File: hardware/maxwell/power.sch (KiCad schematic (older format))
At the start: 30 parts, among them J7 Dynamo Input, J9 Battery, Q2 PSMN5R4-25YLD, Q3 NTR1P02T1, Q4 NTR1P02T1, Q5 NTR1P02T1, U10 MIC39102, U8 TLP188, U9 Buck Regulator

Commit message: Updating for manufacture.
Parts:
- removed C15: 100u, coddingtonbear:CP_Tantalum_Case-D_EIA-7343-31_Milling, symbol maxwell-rescue:CP-RESCUE-maxwell
- removed D2, D3: 18, adamgreig/agg-kicad/agg.pretty:DO-214AA-SMB, symbol maxwell-rescue:D_Zener-RESCUE-maxwell
- removed R34: 110k, coddingtonbear/coddingtonbear.pretty:0805_Milling, symbol maxwell-rescue:R-RESCUE-maxwell
- removed R35: 10k, coddingtonbear/coddingtonbear.pretty:0805_Milling, symbol maxwell-rescue:R-RESCUE-maxwell
- added D2: GS1M-LTP, mcous/kicad-lib/footprints/diode.pretty:DO-214AC, symbol pspice:DIODE
- added J18: Supercap, coddingtonbear/coddingtonbear.pretty:JST_XH_B02B-XH-A_02x2.50mm_Straight_LargePads, symbol maxwell-rescue:Conn_01x02-RESCUE-maxwell
- added Q6: NTR1P02T1, coddingtonbear/coddingtonbear.pretty:SOT-23_LargePads, symbol device:Q_PMOS_GSD
- added R15: 10k, coddingtonbear/coddingtonbear.pretty:0805_Milling, symbol maxwell-rescue:R-RESCUE-maxwell
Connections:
- net labels added: BATT_SOURCE_DISABLE, VCC
- net labels removed: DYNAMO_VOLTAGE
- wire segments 85 -> 87
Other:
- note added: "Tune to 5V"
- note removed: "Tune to 4V"
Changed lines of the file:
@@
-$EndComp
-$Comp
-L maxwell-rescue:D_Zener-RESCUE-maxwell D2
-U 1 1 5A1FF2A4
-P 2400 1050
-F 0 "D2" V 2354 1129 50  0000 L CNN
-F 1 "18" V 2445 1129 50  0000 L CNN
-F 2 "adamgreig/agg-kicad/agg.pretty:DO-214AA-SMB" H 2400 1050 50  0001 C CNN
-F 3 "" H 2400 1050 50  0001 C CNN
-	1    2400 1050
-	0    1    1    0
-$EndComp
-$Comp
-L maxwell-rescue:D_Zener-RESCUE-maxwell D3
-U 1 1 5A1FF2AB
-P 2400 1400
-F 0 "D3" V 2446 1321 50  0000 R CNN
-F 1 "18" V 2355 1321 50  0000 R CNN
-F 2 "adamgreig/agg-kicad/agg.pretty:DO-214AA-SMB" H 2400 1400 50  0001 C CNN
-F 3 "" H 2400 1400 50  0001 C CNN
-	1    2400 1400
-	0    -1   -1   0
 $EndComp
 $Comp
@@
 F 3 "" H 5150 1350 50  0001 C CNN
 	1    5150 1350
-	1    0    0    -1
-$EndComp
-$Comp
-L maxwell-rescue:CP-RESCUE-maxwell C15
-U 1 1 5A20260D
-P 3650 1600
-F 0 "C15" H 3768 1646 50  0000 L CNN
-F 1 "100u" H 3768 1555 50  0000 L CNN
-F 2 "coddingtonbear:CP_Tantalum_Case-D_EIA-7343-31_Milling" H 3688 1450 50  0001 C CNN
-F 3 "" H 3650 1600 50  0001 C CNN
-	1    3650 1600
-	1    0    0    -1
-$EndComp
-$Comp
-L maxwell-rescue:GND-RESCUE-maxwell #PWR040
-U 1 1 5A202661
-P 3650 1750
-F 0 "#PWR040" H 3650 1500 50  0001 C CNN
-F 1 "GND" H 3655 1577 50  0000 C CNN
-F 2 "" H 3650 1750 50  0001 C CNN
-F 3 "" H 3650 1750 50  0001 C CNN
-	1    3650 1750
 	1    0    0    -1
 $EndComp
@@
 ~BATT_CHARGING
 Text Notes 4400 1550 0    60   ~ 0
-Tune to 4V
+Tune to 5V
 $Comp
 L maxwell-rescue:C-RESCUE-maxwell C18
@@
 ~BATT_CHARGE_ENABLE
 $Comp
-L maxwell-rescue:R-RESCUE-maxwell R34
-U 1 1 5A27817C
-P 4150 850
-F 0 "R34" H 4220 896 50  0000 L CNN
-F 1 "110k" H 4220 805 50  0000 L CNN
-F 2 "coddingtonbear/coddingtonbear.pretty:0805_Milling" V 4080 850 50  0001 C CNN
-F 3 "" H 4150 850 50  0001 C CNN
-	1    4150 850
-	0    -1   -1   0
-$EndComp
-$Comp
-L maxwell-rescue:R-RESCUE-maxwell R35
-U 1 1 5A2781E1
-P 4500 850
-F 0 "R35" H 4570 896 50  0000 L CNN
-F 1 "10k" H 4570 805 50  0000 L CNN
-F 2 "coddingtonbear/coddingtonbear.pretty:0805_Milling" V 4430 850 50  0001 C CNN
-F 3 "" H 4500 850 50  0001 C CNN
-	1    4500 850
-	0    -1   -1   0
-$EndComp
-$Comp
-L maxwell-rescue:GND-RESCUE-maxwell #PWR046
-U 1 1 5A278243
-P 4650 850
-F 0 "#PWR046" H 4650 600 50  0001 C CNN
-F 1 "GND" H 4655 677 50  0000 C CNN
-F 2 "" H 4650 850 50  0001 C CNN
-F 3 "" H 4650 850 50  0001 C CNN
-	1    4650 850
-	0    -1   -1   0
-$EndComp
-Text GLabel 4400 650  2    60   Output ~ 0
-DYNAMO_VOLTAGE
-$Comp
 L maxwell-rescue:+BATT-RESCUE-maxwell #PWR043
 U 1 1 5A210C7A
@@
 $EndComp
 Wire Wire Line
-	2400 1250 2400 1200
-Wire Wire Line
-	1300 900  2400 900
-Wire Wire Line
-	1300 1550 2400 1550
-Wire Wire Line
 	3350 900  3350 950
-Connection ~ 2400 900
-Connection ~ 2400 1550
-Wire Wire Line
-	3650 1250 3650 1450
-Wire Wire Line
-	3650 1250 3800 1250
 Wire Wire Line
 	5600 1250 5650 1250
@@
 Connection ~ 10100 2150
 Wire Wire Line
-	5650 1600 5650 2000
+	5650 1600 5650 1900
 Wire Wire Line
 	5650 2000 5900 2000
@@
 Wire Wire Line
 	1500 3500 1350 3500
-Wire Wire Line
-	4000 850  3800 850
-Wire Wire Line
-	3800 850  3800 1250
-Connection ~ 3800 1250
-Wire Wire Line
-	4300 850  4350 850
-Wire Wire Line
-	4300 850  4300 650
-Wire Wire Line
-	4300 650  4400 650
 Wire Wire Line
 	5200 1250 5150 1250
@@
 DYNAMO_AC
 Wire Wire Line
-	2400 900  3350 900
-Wire Wire Line
-	2400 1550 3350 1550
-Wire Wire Line
 	5900 1250 6400 1250
 Wire Wire Line
@@
 Wire Wire Line
 	5900 2000 5900 2050
-Wire Wire Line
-	3800 1250 4200 1250
 Wire Wire Line
 	7350 1800 7450 1800
@@
 L maxwell-rescue:+BATT-RESCUE-maxwell #PWR037
 U 1 1 5A884C49
-P 4950 2850
-F 0 "#PWR037" H 4950 2700 50  0001 C CNN
-F 1 "+BATT" H 4965 3023 50  0000 C CNN
-F 2 "" H 4950 2850 50  0001 C CNN
-F 3 "" H 4950 2850 50  0001 C CNN
-	1    4950 2850
+P 4950 2450
+F 0 "#PWR037" H 4950 2300 50  0001 C CNN
+F 1 "+BATT" H 4965 2623 50  0000 C CNN
+F 2 "" H 4950 2450 50  0001 C CNN
+F 3 "" H 4950 2450 50  0001 C CNN
+	1    4950 2450
 	1    0    0    -1
 $EndComp
@@
 	8250 1350 8400 1350
 Connection ~ 8250 1250
+$Comp
+L device:Q_PMOS_GSD Q6
+U 1 1 5B30AA5F
+P 4850 2650
+F 0 "Q6" V 5100 2650 50  0000 C CNN
+F 1 "NTR1P02T1" V 5191 2650 50  0000 C CNN
+F 2 "coddingtonbear/coddingtonbear.pretty:SOT-23_LargePads" H 5050 2750 50  0001 C CNN
+F 3 "" H 4850 2650 50  0001 C CNN
+	1    4850 2650
+	1    0    0    -1
+$EndComp
+Wire Wire Line
+	5200 1250 5200 1700
+Connection ~ 5200 1250
+$Comp
+L pspice:DIODE D2
+U 1 1 5B30CFBF
+P 4150 2500
+F 0 "D2" V 4104 2628 50  0000 L CNN
+F 1 "GS1M-LTP" V 4195 2628 50  0000 L CNN
+F 2 "mcous/kicad-lib/footprints/diode.pretty:DO-214AC" H 4150 2500 50  0001 C CNN
+F 3 "" H 4150 2500 50  0001 C CNN
+	1    4150 2500
+	0    1    1    0
+$EndComp
+Wire Wire Line
+	4150 1700 5200 1700
+Wire Wire Line
+	4150 1700 4150 2300
+$Comp
+L maxwell-rescue:R-RESCUE-maxwell R15
+U 1 1 5B31404F
+P 4800 1900
+F 0 "R15" V 5007 1900 50  0000 C CNN
+F 1 "10k" V 4916 1900 50  0000 C CNN
+F 2 "coddingtonbear/coddingtonbear.pretty:0805_Milling" V 4730 1900 50  0001 C CNN
+F 3 "" H 4800 1900 50  0001 C CNN
+	1    4800 1900
+	0    1    1    0
+$EndComp
+Wire Wire Line
+	4950 1900 5650 1900
+Connection ~ 5650 1900
+Wire Wire Line
+	5650 1900 5650 2000
+Wire Wire Line
+	1300 900  3350 900
+Wire Wire Line
+	1300 1550 3350 1550
+Text GLabel 4400 2200 3    60   Input ~ 0
+BATT_SOURCE_DISABLE
+Wire Wire Line
+	4650 1900 4650 2650
+Wire Wire Line
+	4400 2200 4400 1900
+Wire Wire Line
+	4400 1900 4650 1900
+Connection ~ 4650 1900
+Wire Wire Line
+	4150 3400 4600 3400
+Wire Wire Line
+	4600 3400 4600 2850
+Wire Wire Line
+	4600 2850 4950 2850
+Wire Wire Line
+	4150 2700 4150 3400
+$Comp
+L power:VCC #PWR0103
+U 1 1 5B32131C
+P 5250 2850
+F 0 "#PWR0103" H 5250 2700 50  0001 C CNN
+F 1 "VCC" H 5267 3023 50  0000 C CNN
+F 2 "" H 5250 2850 50  0001 C CNN
+F 3 "" H 5250 2850 50  0001 C CNN
+	1    5250 2850
+	1    0    0    -1
+$EndComp
+Connection ~ 5250 2850
+Wire Wire Line
+	3650 1250 4200 1250
+$Comp
+L maxwell-rescue:Conn_01x02-RESCUE-maxwell J18
+U 1 1 5B33B354
+P 6250 4150
+F 0 "J18" H 6330 4142 50  0000 L CNN
+F 1 "Supercap" H 6330 4051 50  0000 L CNN
+F 2 "coddingtonbear/coddingtonbear.pretty:JST_XH_B02B-XH-A_02x2.50mm_Straight_LargePads" H 6250 4150 50  0001 C CNN
+F 3 "" H 6250 4150 50  0001 C CNN
+	1    6250 4150
+	0    1    1    0
+$EndComp
+$Comp
+L maxwell-rescue:GND-RESCUE-maxwell #PWR0111
+U 1 1 5B33B419
+P 6250 3950
+F 0 "#PWR0111" H 6250 3700 50  0001 C CNN
+F 1 "GND" H 6255 3777 50  0000 C CNN
+F 2 "" H 6250 3950 50  0001 C CNN
+F 3 "" H 6250 3950 50  0001 C CNN
+	1    6250 3950
+	-1   0    0    1
+$EndComp
+$Comp
+L maxwell-rescue:+3V3-RESCUE-maxwell #PWR0112
+U 1 1 5B33B498
+P 6150 3950
+F 0 "#PWR0112" H 6150 3800 50  0001 C CNN
+F 1 "+3V3" H 6165 4123 50  0000 C CNN
+F 2 "" H 6150 3950 50  0001 C CNN
+F 3 "" H 6150 3950 50  0001 C CNN
+	1    6150 3950
+	1    0    0    -1
+$EndComp
 $EndSCHEMATC

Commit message: Updating hardware design.
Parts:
- Q2: symbol device:Q_NMOS_SGD -> maxwell-rescue:Q_NMOS_SGD-device
- Q3, Q4, Q5, Q6: symbol device:Q_PMOS_GSD -> maxwell-rescue:Q_PMOS_GSD-device
- U10: symbol coddingtonbear:MIC39102 -> maxwell-rescue:MIC39102-coddingtonbear
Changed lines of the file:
@@
 	9900 1100 9900 1800
 $Comp
-L device:Q_PMOS_GSD Q4
+L maxwell-rescue:Q_PMOS_GSD-device Q4
 U 1 1 5A85109E
 P 7850 1350
@@
 $EndComp
 $Comp
-L device:Q_PMOS_GSD Q3
+L maxwell-rescue:Q_PMOS_GSD-device Q3
 U 1 1 5A876381
 P 5400 1150
@@
 $EndComp
 $Comp
-L device:Q_NMOS_SGD Q2
+L maxwell-rescue:Q_NMOS_SGD-device Q2
 U 1 1 5A87E051
 P 3150 3900
@@
 $EndComp
 $Comp
-L coddingtonbear:MIC39102 U10
+L maxwell-rescue:MIC39102-coddingtonbear U10
 U 1 1 5A881E0A
 P 6150 3100
@@
 $EndComp
 $Comp
-L device:Q_PMOS_GSD Q5
+L maxwell-rescue:Q_PMOS_GSD-device Q5
 U 1 1 5A851232
 P 9200 1200
@@
 Connection ~ 8250 1250
 $Comp
-L device:Q_PMOS_GSD Q6
+L maxwell-rescue:Q_PMOS_GSD-device Q6
 U 1 1 5B30AA5F
 P 4850 2650

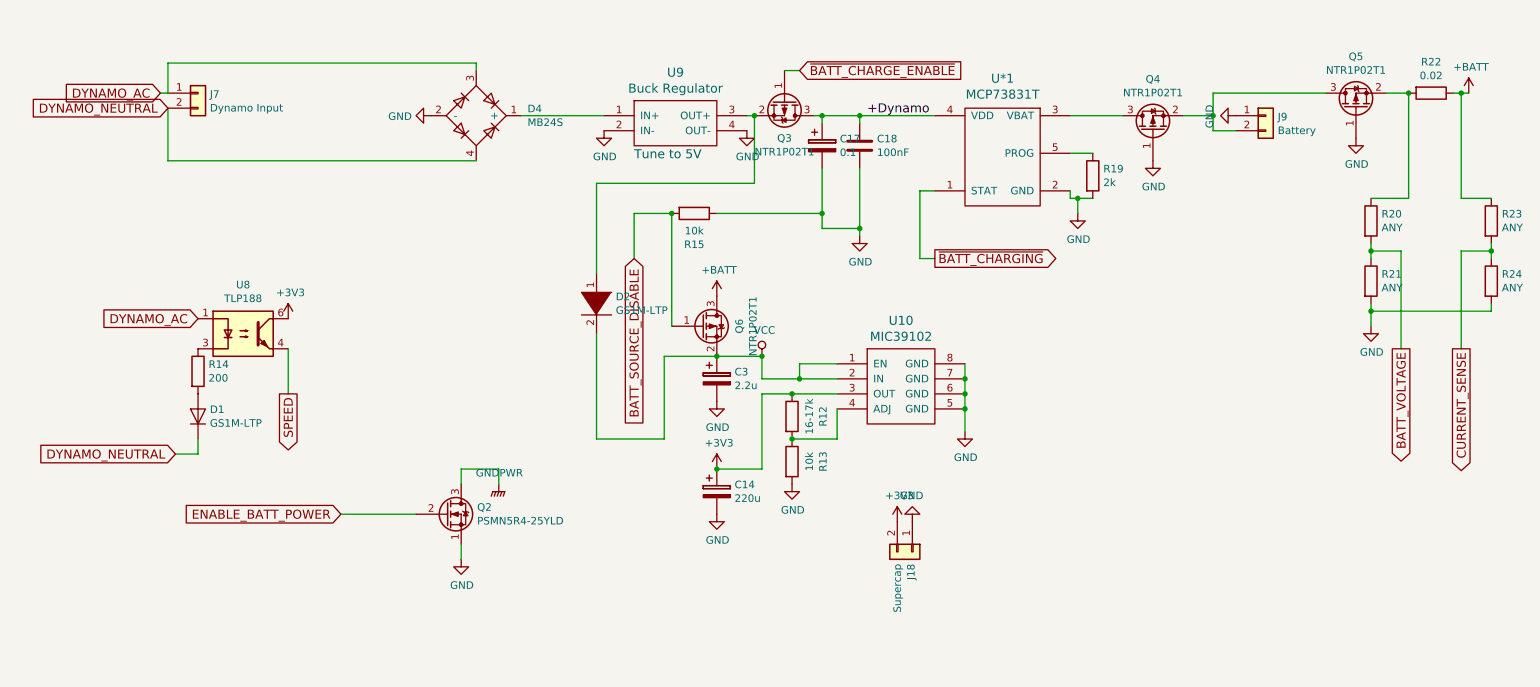
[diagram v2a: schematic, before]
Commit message: Preparing maxwell hardware for next revision.
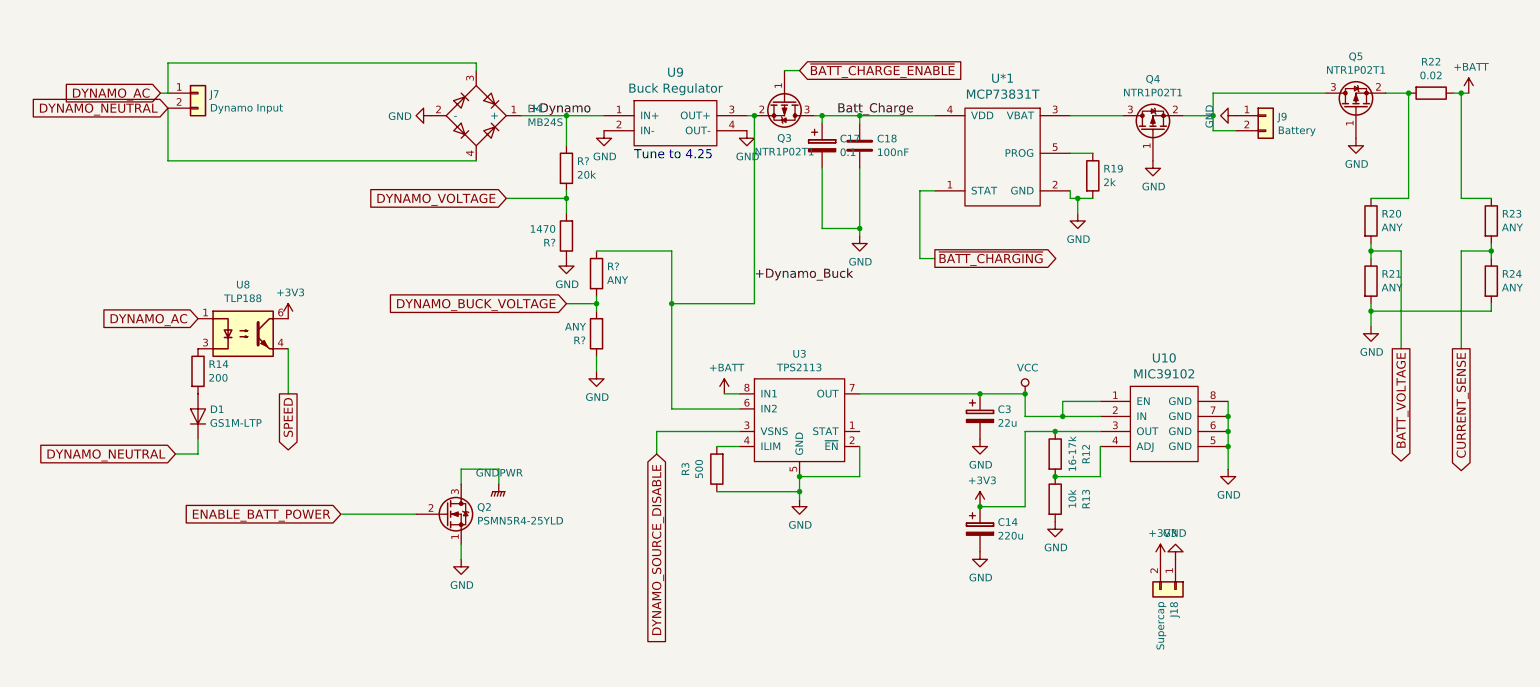
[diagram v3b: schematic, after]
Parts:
- removed D2: GS1M-LTP, mcous/kicad-lib/footprints/diode.pretty:DO-214AC, symbol pspice:DIODE
- removed Q6: NTR1P02T1, coddingtonbear/coddingtonbear.pretty:SOT-23_LargePads, symbol maxwell-rescue:Q_PMOS_GSD-device
- removed R15: 10k, coddingtonbear/coddingtonbear.pretty:0805_Milling, symbol maxwell-rescue:R-RESCUE-maxwell
- added R3: 500, coddingtonbear/coddingtonbear.pretty:0805_Milling, symbol maxwell-rescue:R-RESCUE-maxwell
- added R? (x2): ANY, coddingtonbear/coddingtonbear.pretty:0805_Milling, symbol maxwell-rescue:R-RESCUE-maxwell
- added R?: 20k, coddingtonbear/coddingtonbear.pretty:0805_Milling, symbol maxwell-rescue:R-RESCUE-maxwell
- added R?: 1470, coddingtonbear/coddingtonbear.pretty:0805_Milling, symbol maxwell-rescue:R-RESCUE-maxwell
- added U3: TPS2113, Package_SO:TSSOP-8_4.4x3mm_P0.65mm, symbol coddingtonbear:TPS2113
- C3: value 2.2u -> 22u
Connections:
- net +BATT: now also U3.8 (IN1)
- net +Dynamo: now also D4.1 (+), U9.1 (IN+), R?.1; no longer C17.1, C18.2, Q3.3 (D), U*1.4 (VDD)
- net GND: now also R3.1, R?.1, R?.1, U3.2 (~EN), U3.5 (GND)
- net VCC: now also U3.7 (OUT)
- net +Dynamo_Buck: now reaches Q3.2 (S), U9.3 (OUT+)
- net +Dynamo_Buck: now also R?.1, U3.6 (IN2)
- new net: R3.2, U3.4 (ILIM)
- new net Batt_Charge: C17.1, C18.2, Q3.3 (D), U*1.4 (VDD)
- new net DYNAMO_BUCK_VOLTAGE: R?.2, R?.2
- new net DYNAMO_SOURCE_DISABLE: U3.3 (VSNS)
- new net DYNAMO_VOLTAGE: R?.2, R?.2
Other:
- note added: "Tune to 4.25"
- note removed: "Tune to 5V"
- moved on the sheet: C14, C3, J18, R12, R13, U10
